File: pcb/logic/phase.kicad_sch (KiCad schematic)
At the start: 2 parts, among them J1 Conn_02x02_Odd_Even, J2 Conn_02x03_Odd_Even

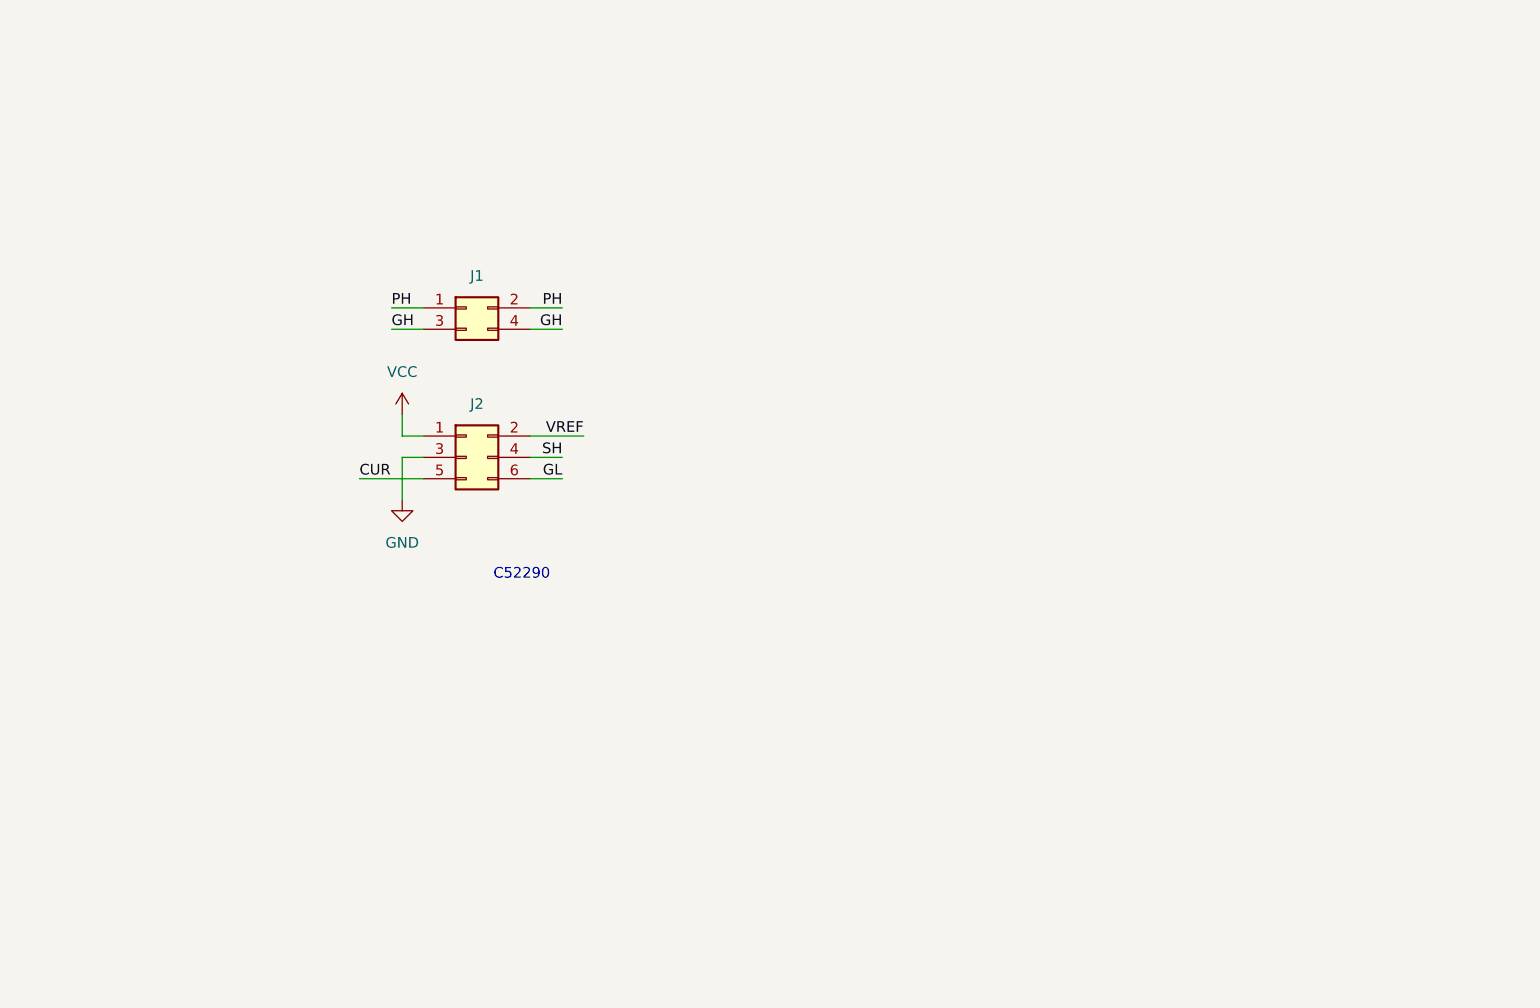
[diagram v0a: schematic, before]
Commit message: Finish rev 1
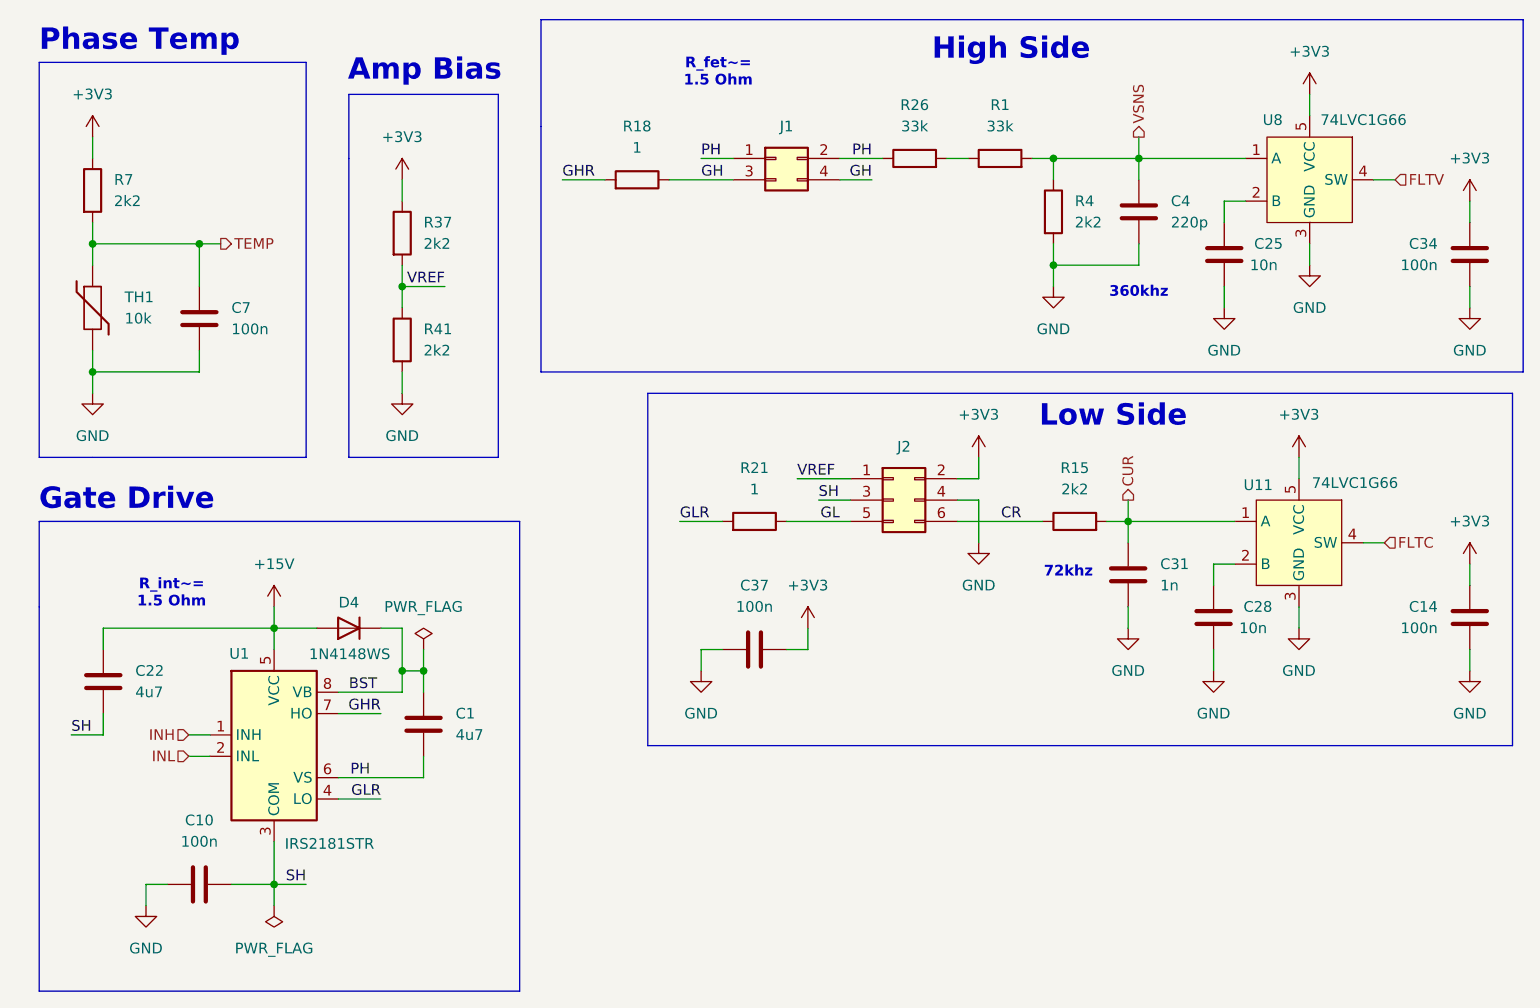
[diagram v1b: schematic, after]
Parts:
- added C1: 4u7, Capacitor_SMD:C_1206_3216Metric, symbol Device:C
- added C10, C14, C34, C37, C7: 100n, Capacitor_SMD:C_0402_1005Metric, symbol Device:C
- added C22: 4u7, Capacitor_SMD:C_0805_2012Metric, symbol Device:C
- added C25, C28: 10n, Capacitor_SMD:C_0402_1005Metric, symbol Device:C
- added C31: 1n, Capacitor_SMD:C_0402_1005Metric, symbol Device:C
- added C4: 220p, Capacitor_SMD:C_0402_1005Metric, symbol Device:C
- added D4: 1N4148WS, Diode_SMD:D_SOD-323, symbol Diode:1N4148WS
- added R1, R26: 33k, Resistor_SMD:R_0402_1005Metric, symbol Device:R
- added R15, R37, R4, R41, R7: 2k2, Resistor_SMD:R_0402_1005Metric, symbol Device:R
- added R18, R21: 1, Resistor_SMD:R_0603_1608Metric, symbol Device:R
- added TH1: 10k, Resistor_SMD:R_0402_1005Metric, symbol Device:Thermistor
- added U1: IRS2181STR, Package_SO:JEITA_SOIC-8_3.9x4.9mm_P1.27mm, symbol User_Symbols:IRS2181STR
- added U11, U8: 74LVC1G66, Package_TO_SOT_SMD:SOT-23-5, symbol User_Symbols:74LVC1G66
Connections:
- net VCC is gone; now on net VREF: J2.1 (Pin_1)
- net CUR: now also C31.1, R15.2, U11.1 (A); no longer J2.5 (Pin_5)
- net GH: now also R18.1
- net GL: now also J2.5 (Pin_5), R21.1; no longer J2.6 (Pin_6)
- net GND: now also J2.4 (Pin_4), C10.1, C14.2, C25.2, C28.2, C31.2, C34.2, C37.1, C4.2, C7.2, R4.2, R41.2, TH1.2, U11.3 (GND), U8.3 (GND); no longer J2.3 (Pin_3)
- net PH: now also C1.2, R26.1, U1.6 (VS)
- net SH: now also J2.3 (Pin_3), C10.2, C22.2, U1.3 (COM); no longer J2.4 (Pin_4)
- net VREF: now also R37.2, R41.1; no longer J2.2 (Pin_2)
- new net: C28.1, U11.2 (B)
- new net: R1.1, R26.2
- new net: C25.1, U8.2 (B)
- new net +15V: C22.1, D4.2 (A), U1.5 (VCC)
- new net +3V3: C14.1, C34.1, C37.2, J2.2 (Pin_2), R37.1, R7.1, U11.5 (VCC), U8.5 (VCC)
- new net BST: C1.1, D4.1 (K), U1.8 (VB)
- new net CR: J2.6 (Pin_6), R15.1
- new net FLTC: U11.4 (SW)
- new net FLTV: U8.4 (SW)
- new net GHR: R18.2, U1.7 (HO)
- new net GLR: R21.2, U1.4 (LO)
- new net INH: U1.1 (INH)
- new net INL: U1.2 (INL)
- new net TEMP: C7.1, R7.2, TH1.1
- new net VSNS: C4.1, R1.2, R4.1, U8.1 (A)
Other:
- note added: "360khz"
- note added: "72khz"
- note added: "Amp Bias"
- note added: "Gate Drive"
- note added: "High Side"
- note added: "Low Side"
- note added: "Phase Temp"
- note added: "R_fet~= 1.5 Ohm"
- note added: "R_int~= 1.5 Ohm"
- note removed: "C52290"
- moved on the sheet: J1, J2
